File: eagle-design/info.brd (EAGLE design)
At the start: 57.2 x 64.4 mm, 17 parts

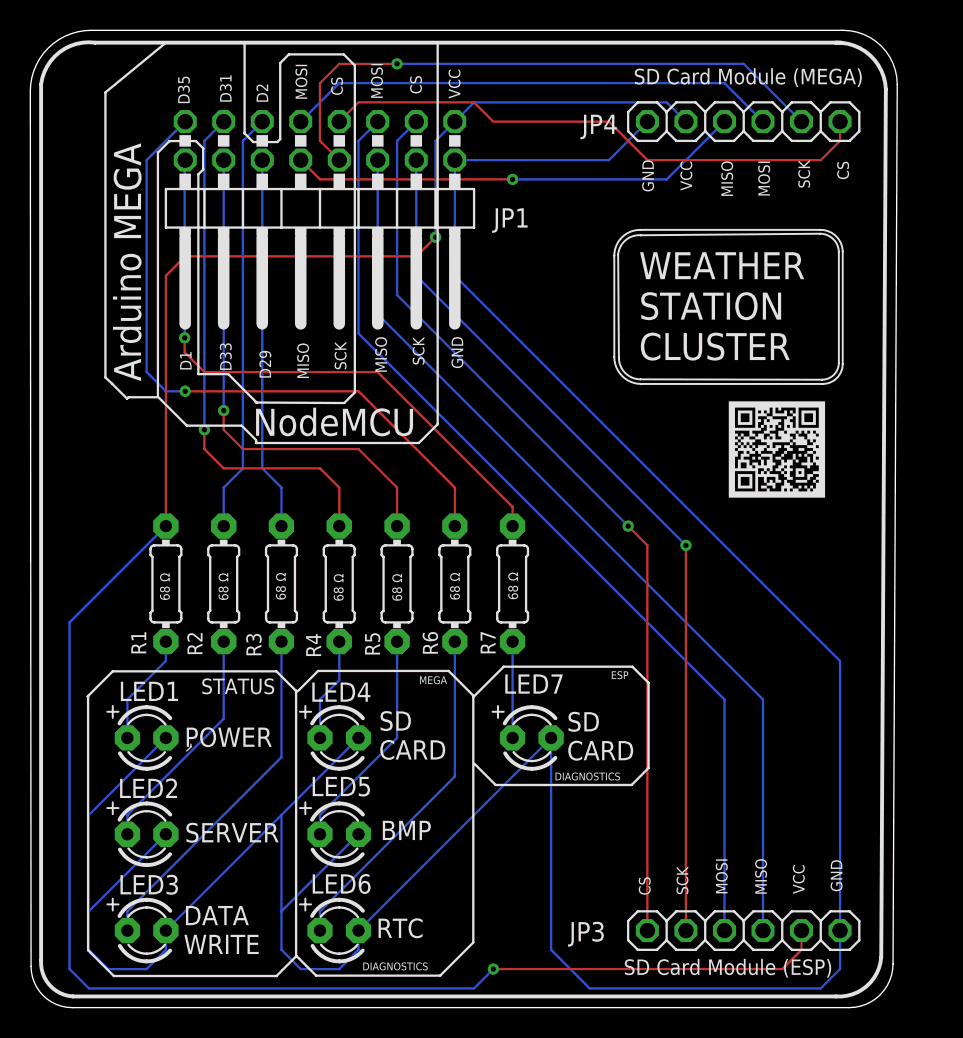
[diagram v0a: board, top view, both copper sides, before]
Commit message: Added new design
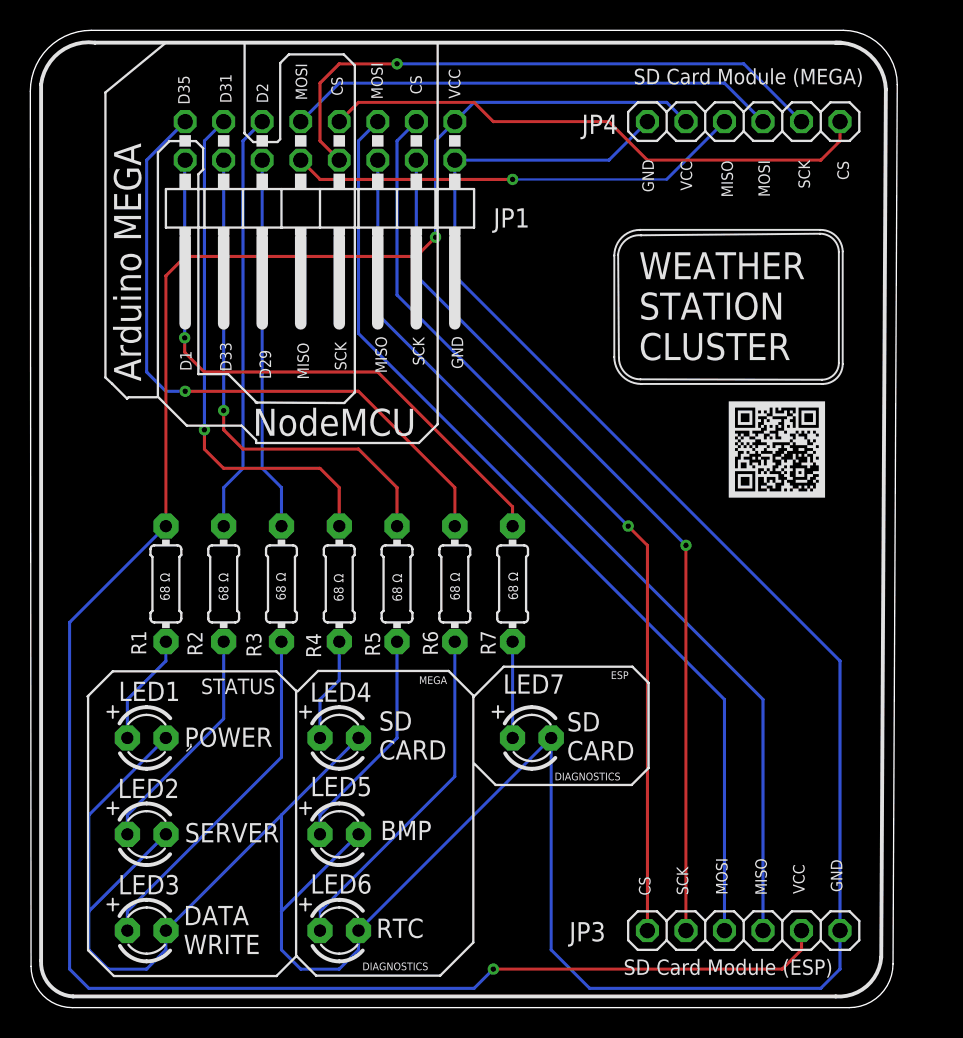
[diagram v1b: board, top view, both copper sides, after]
